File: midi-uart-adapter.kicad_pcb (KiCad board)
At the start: 2 copper layers, 48.3 x 61.6 mm, 25 parts, among them U1 6N138

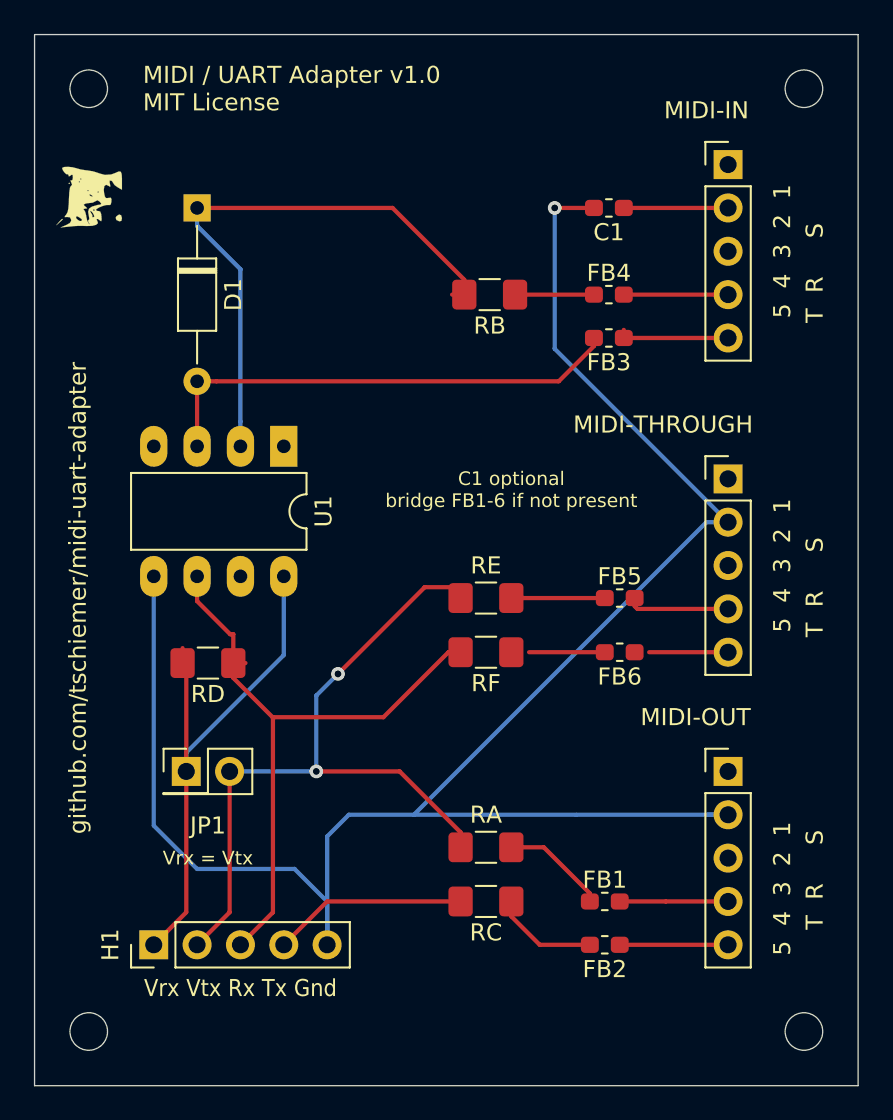
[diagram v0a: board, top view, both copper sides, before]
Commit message: v2.0
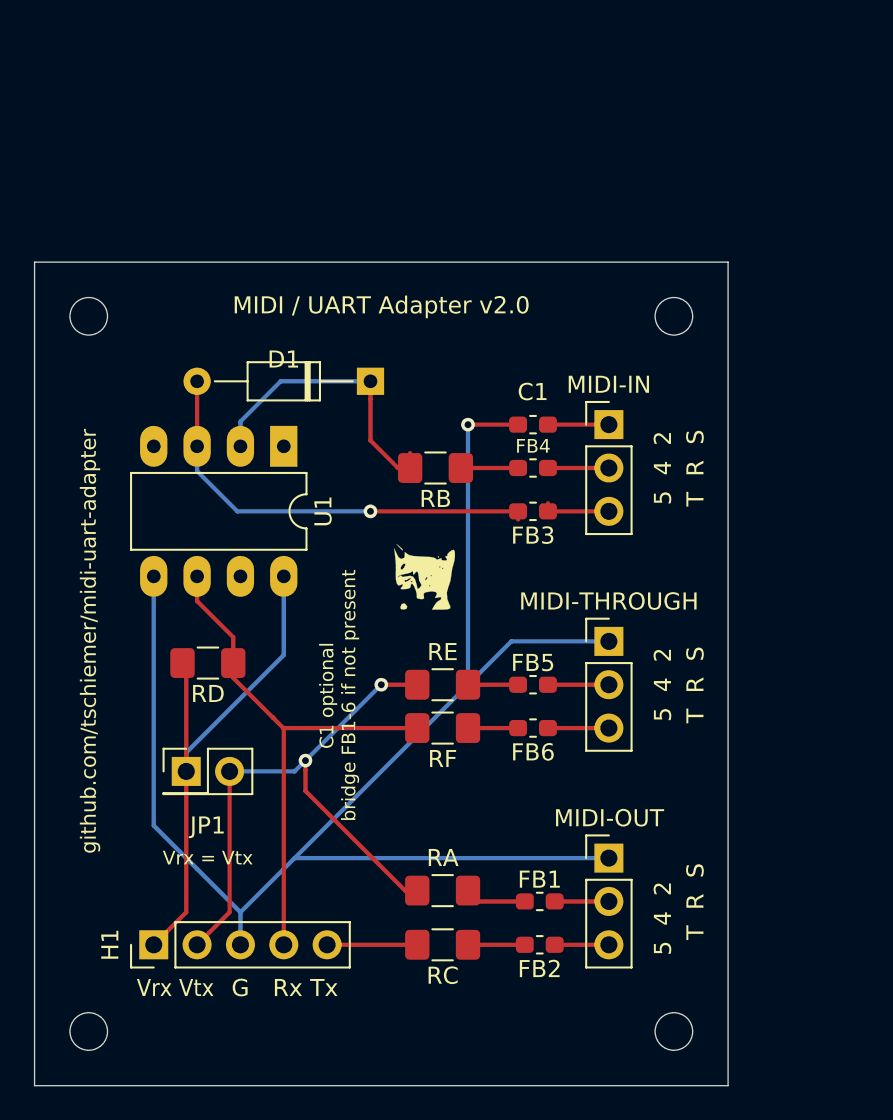
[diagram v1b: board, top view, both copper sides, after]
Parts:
- MIDI-IN, MIDI-OUT, MIDI-THROUGH: footprint Connector_PinHeader_2.54mm:PinHeader_1x05_P2.54mm_Vertical -> Connector_PinHeader_2.54mm:PinHeader_1x03_P2.54mm_Vertical
- moved G*** 29.7 mm to (143.5, 101.6), turned to 0 degrees
- moved MIDI-IN 16.8 mm to (154.3, 92.7)
- moved REF** 15.4 mm to (158.1, 86.4)
- moved D1 14.4 mm to (140.3, 90.2), turned to 180 degrees
- moved C1 13.5 mm to (149.9, 92.7)
- moved REF** 13.3 mm to (123.8, 86.4)
- moved MIDI-THROUGH 11.8 mm to (154.3, 105.4)
- moved FB3 11.1 mm to (149.9, 97.8)
- moved FB4 11.1 mm to (149.9, 95.2)
- moved RB 10.6 mm to (144.1, 95.2)
- moved MIDI-OUT 8.64 mm to (154.3, 118.1)
- moved REF** 7.62 mm to (158.1, 128.3)
- moved FB5 7.18 mm to (149.9, 108.0)
- moved FB6 6.75 mm to (149.9, 110.5)
- moved RE 5.68 mm to (144.6, 108.0)
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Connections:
- C1 pad 1: Net-(C2-Pad1) -> Net-(C1-Pad1)
- H1 pad 3: UART_rx -> GNDREF
- H1 pad 4: UART_tx -> UART_rx
- H1 pad 5: GNDREF -> UART_tx
- MIDI-IN pad 1: Net-(MIDI-IN1-Pad1) -> Net-(C1-Pad1)
- MIDI-IN pad 2: Net-(C2-Pad1) -> Net-(FB4-Pad1)
- MIDI-IN pad 3: Net-(MIDI-IN1-Pad3) -> Net-(FB3-Pad1)
- MIDI-OUT pad 1: Net-(MIDI-OUT1-Pad1) -> GNDREF
- MIDI-OUT pad 2: GNDREF -> Net-(FB1-Pad1)
- MIDI-OUT pad 3: Net-(MIDI-OUT1-Pad3) -> Net-(FB2-Pad1)
- MIDI-THROUGH pad 1: Net-(MIDI-THROUGH1-Pad1) -> GNDREF
- MIDI-THROUGH pad 2: GNDREF -> Net-(FB5-Pad1)
- MIDI-THROUGH pad 3: Net-(MIDI-THROUGH1-Pad3) -> Net-(FB6-Pad1)
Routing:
- net GNDREF: track 112.4 -> 88.4 mm
- net Net-(D1-Pad1): track 34.0 -> 17.4 mm
- net VCC_tx: track 42.4 -> 34.8 mm
- net UART_tx: track 11.4 -> 5.28 mm
- net Net-(C2-Pad1): track 6.11 -> 0.00 mm
- net UART_rx: track 37.6 -> 31.6 mm
- net Net-(FB1-Pad1): track 6.35 -> 2.70 mm
- net Net-(C1-Pad1): track 0.00 -> 3.57 mm
- net Net-(FB1-Pad2): track 6.82 -> 3.59 mm
- net Net-(FB2-Pad1): track 6.35 -> 3.18 mm
- net Net-(D1-Pad2): track 28.4 -> 25.5 mm, vias 0 -> 1
- net Net-(FB2-Pad2): track 6.16 -> 3.33 mm
- net Net-(FB4-Pad1): track 6.11 -> 3.57 mm
- net Net-(FB3-Pad1): track 6.58 -> 4.05 mm
- net Net-(FB5-Pad1): track 6.02 -> 3.57 mm
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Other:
- board size 48.3 x 61.6 mm -> 40.6 x 48.3 mm
- board text added: "5 4 2"
- board text added: "G"
- board text added: "MIDI / UART Adapter v2.0"
- board text added: "Rx Tx"
- board text added: "Vrx Vtx"
- board text removed: "5 4 3 2 1"
- board text removed: "MIDI / UART Adapter v1.0 MIT License"
- board text removed: "Vrx Vtx Rx Tx Gnd"
